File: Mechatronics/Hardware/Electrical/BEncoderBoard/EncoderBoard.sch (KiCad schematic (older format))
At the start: 46 parts, among them IC1 RN4020-V_RM120, IC2 TP4056, IC3 DW01+G, J1 Conn_01x07_Male, J4 Barrel_Jack_Switch, J5 Batt+, J7 Batt-, Q1 FS8205, Q2 Q_PMOS_GSD, Q3 Q_PMOS_GSD, U1 STM32F103C8T6, U2 ITR1802A, U3 ITR1802B, U5 SSD1306OLED, U6 LTC2430, Y1 8Mhz

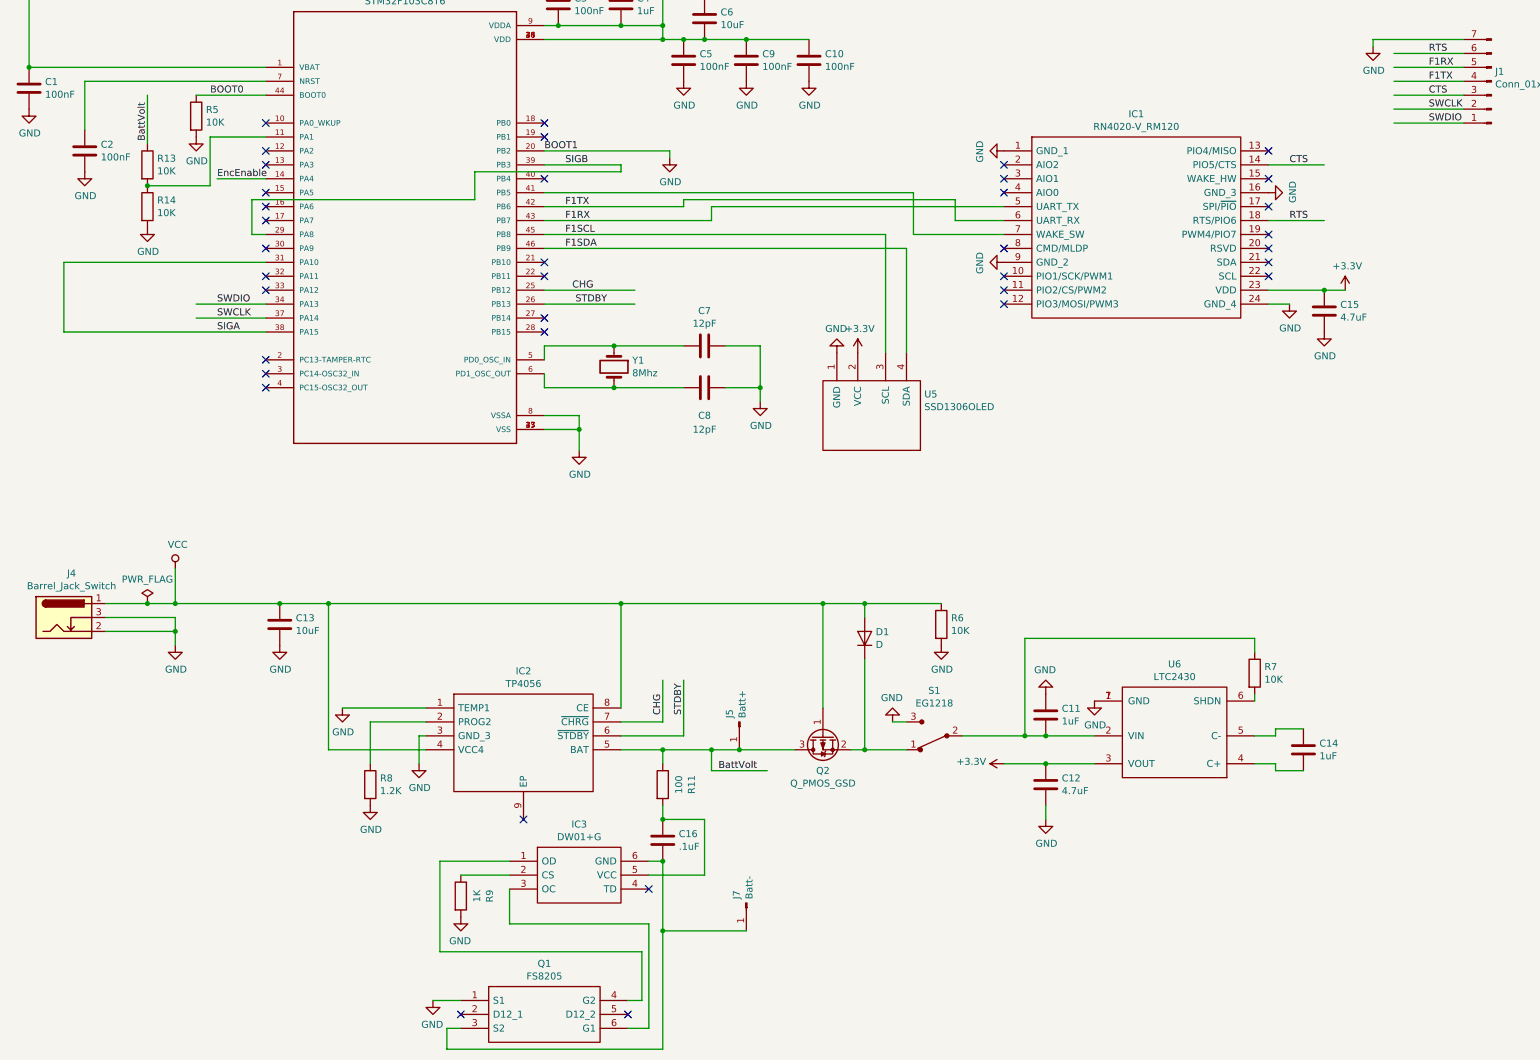
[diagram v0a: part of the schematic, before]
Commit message: Added changes
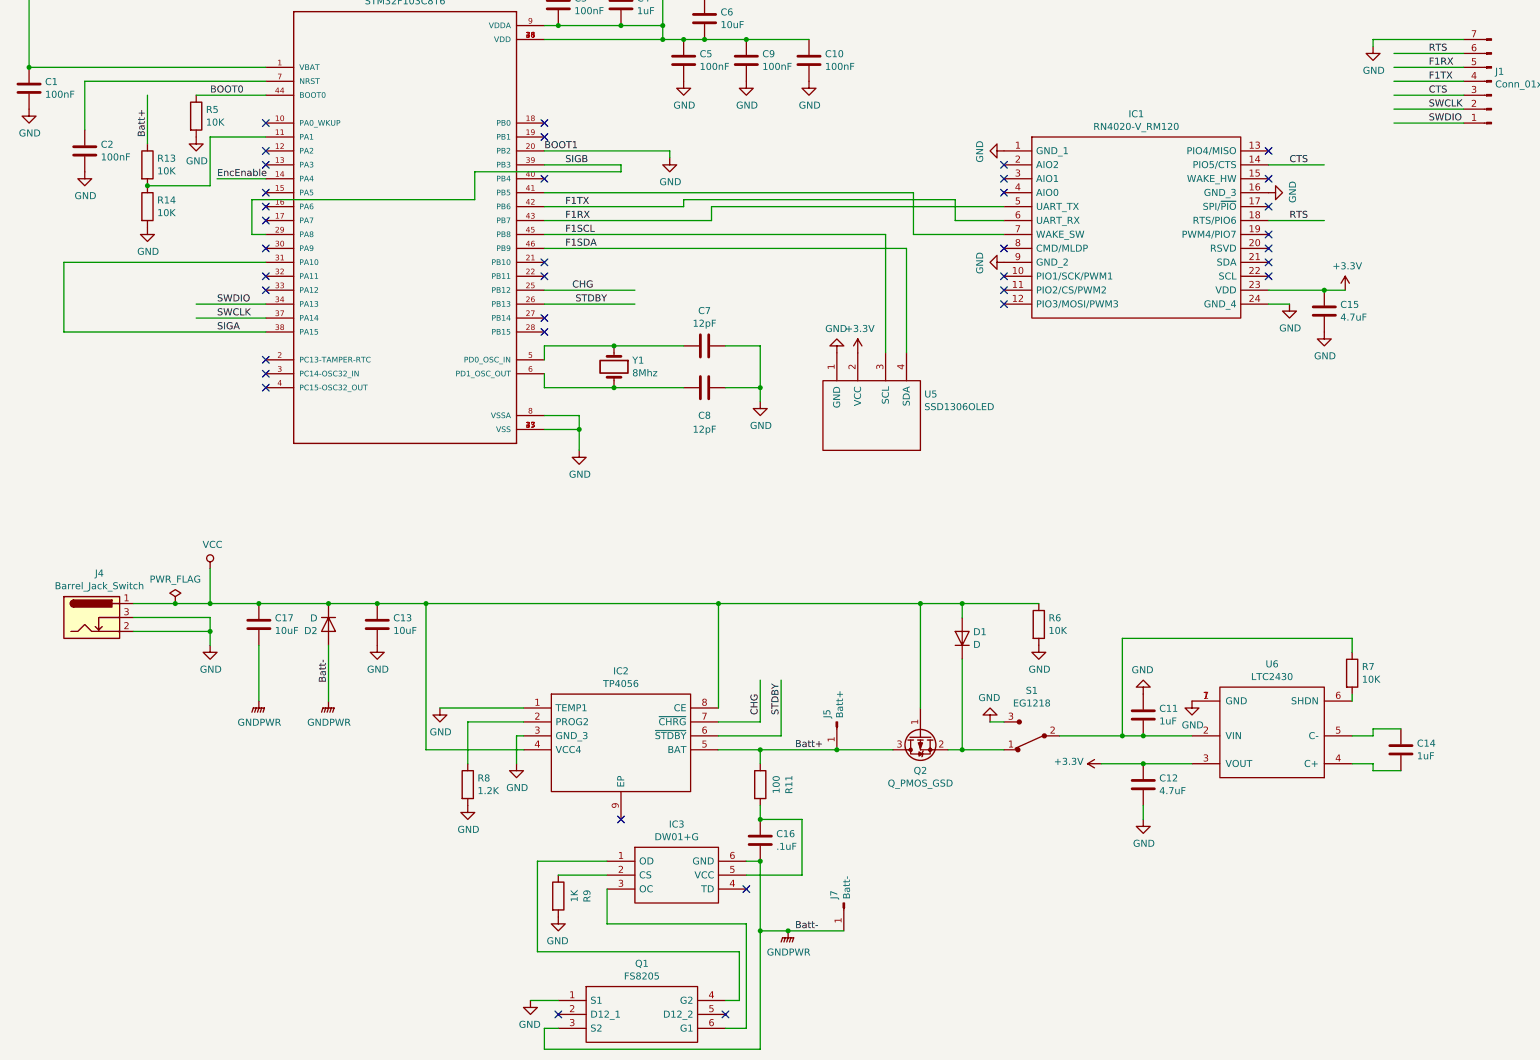
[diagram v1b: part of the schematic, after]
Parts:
- added C17: 10uF, Encoder:C_0603_1608Metric_Pad1.05x0.95mm_HandSolder, symbol Device:C
- added D2: D, Encoder:D_SMA, symbol Device:D
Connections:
- net labels added: Batt+, Batt-, GNDPWR
- net labels removed: BattVolt
- wire segments 175 -> 177
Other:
- moved on the sheet: C11, C12, C13, C14, C16, D1, IC2, IC3, J4, J5, J7, Q1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
